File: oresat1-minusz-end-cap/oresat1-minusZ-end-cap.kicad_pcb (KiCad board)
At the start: 4 copper layers, 105.6 x 105.6 mm, 47 parts, among them J1 M55-7011242R, J2 U.FL-R-SMA, U1 RM3100, U2 RM3100

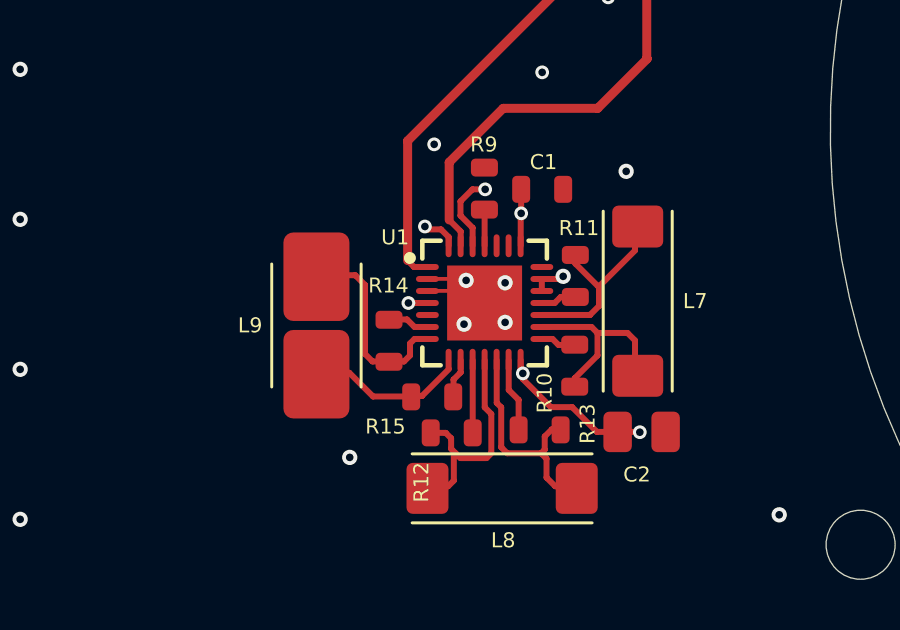
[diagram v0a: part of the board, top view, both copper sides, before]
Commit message: Small changes
Requires layout work still
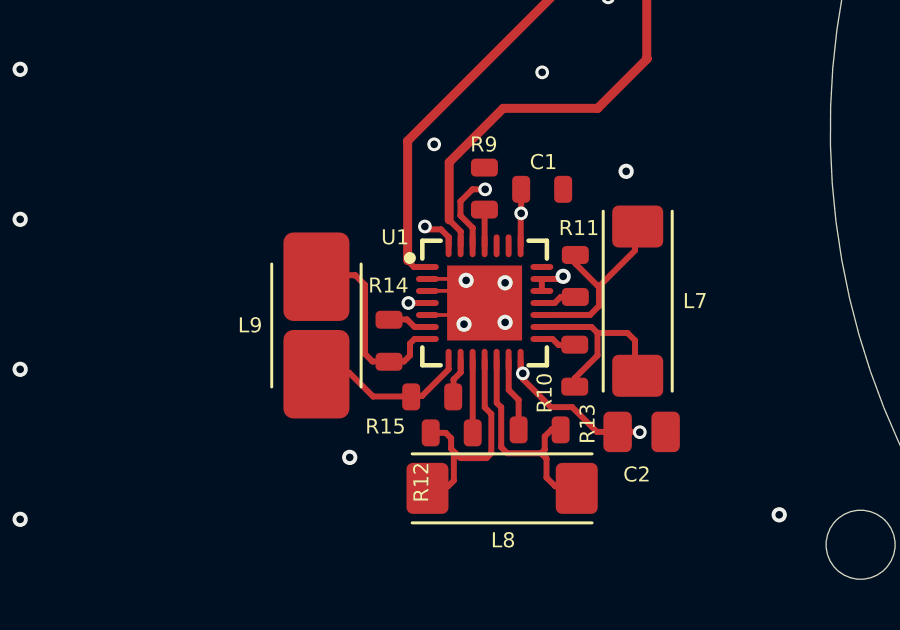
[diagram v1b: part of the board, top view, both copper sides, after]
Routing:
- net GND: track 15.8 -> 17.4 mm
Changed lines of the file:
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@@
 	(gr_arc
 		(start 101.6 64.725)
-		(mid 101.228026 65.623026)
+		(mid 101.228026 65.623025)
 		(end 100.330001 65.995)
 		(stroke
@@
 	(gr_arc
 		(start 107.6 62.825)
-		(mid 107.228026 63.723026)
+		(mid 107.228026 63.723025)
 		(end 106.330001 64.095)
 		(stroke
@@
 	(gr_arc
 		(start 109.5 56.825)
-		(mid 109.128026 57.723026)
+		(mid 109.128026 57.723025)
 		(end 108.230001 58.095)
 		(stroke
@@
 	(gr_arc
 		(start 112.29619 126.860019)
-		(mid 112.674261 126.64133)
+		(mid 112.674262 126.641343)
 		(end 113.104057 126.56364)
 		(stroke
@@
 	(gr_arc
 		(start 113.1115 141.411036)
-		(mid 112.673746 141.333166)
+		(mid 112.673742 141.333171)
 		(end 112.289654 141.109182)
 		(stroke
@@
 	(gr_arc
 		(start 144.8238 146.035212)
-		(mid 145.568657 146.276557)
+		(mid 145.568637 146.276566)
 		(end 146.030398 146.908883)
 		(stroke
@@
 	(gr_arc
 		(start 147.93046 148.284743)
-		(mid 146.757512 147.904661)
+		(mid 146.757527 147.904647)
 		(end 146.030398 146.908883)
 		(stroke
@@
 	(gr_arc
 		(start 150.969602 146.908883)
-		(mid 150.242419 147.904699)
+		(mid 150.242422 147.904669)
 		(end 149.0694 148.284724)
 		(stroke
@@
 	(gr_arc
 		(start 162.940355 125.6597)
-		(mid 162.995109 125.432237)
+		(mid 162.995088 125.432227)
 		(end 163.147407 125.254651)
 		(stroke
@@
 	(gr_arc
 		(start 183.8884 126.56364)
-		(mid 184.322203 126.640035)
+		(mid 184.322207 126.64003)
 		(end 184.703815 126.860023)
 		(stroke
@@
 	(gr_arc
 		(start 184.703946 141.114544)
-		(mid 184.318663 141.335886)
+		(mid 184.31866 141.335883)
 		(end 183.880724 141.411036)
 		(stroke
@@
 	(gr_arc
 		(start 188.77 58.095)
-		(mid 187.871974 57.723026)
+		(mid 187.871975 57.723026)
 		(end 187.5 56.825001)
 		(stroke
@@
 	(gr_arc
 		(start 190.67 64.095)
-		(mid 189.771974 63.723026)
+		(mid 189.771975 63.723026)
 		(end 189.4 62.825001)
 		(stroke
@@
 	(gr_arc
 		(start 191.117776 135.1497)
-		(mid 190.996921 135.690448)
+		(mid 190.996907 135.690432)
 		(end 190.657332 136.128266)
 		(stroke
@@
 	(gr_arc
 		(start 196.67 65.995)
-		(mid 195.771974 65.623026)
+		(mid 195.771975 65.623026)
 		(end 195.4 64.725001)
 		(stroke
@@
 		(width 0.127)
 		(layer "F.Cu")
+		(net "GND")
+	)
+	(segment
+		(start 110.073946 111.188553)
+		(end 111.581446 111.188553)
+		(width 0.127)
+		(layer "F.Cu")
